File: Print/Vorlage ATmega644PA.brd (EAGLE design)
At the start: 84 x 45 mm, 58 parts, among them IC1 ATmega644PA, IC4 ATTINY24/44/84-SSU, Q1 16MHz

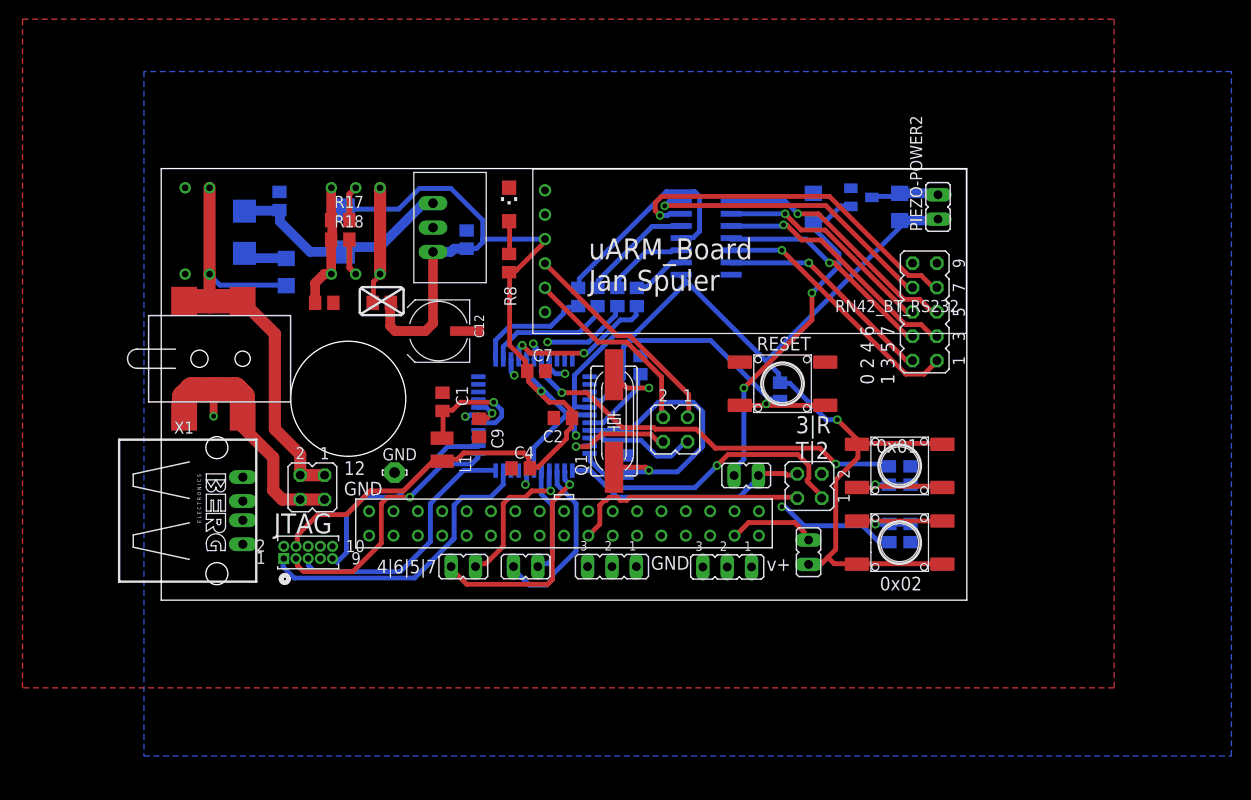
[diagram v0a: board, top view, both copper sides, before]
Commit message: print fertig
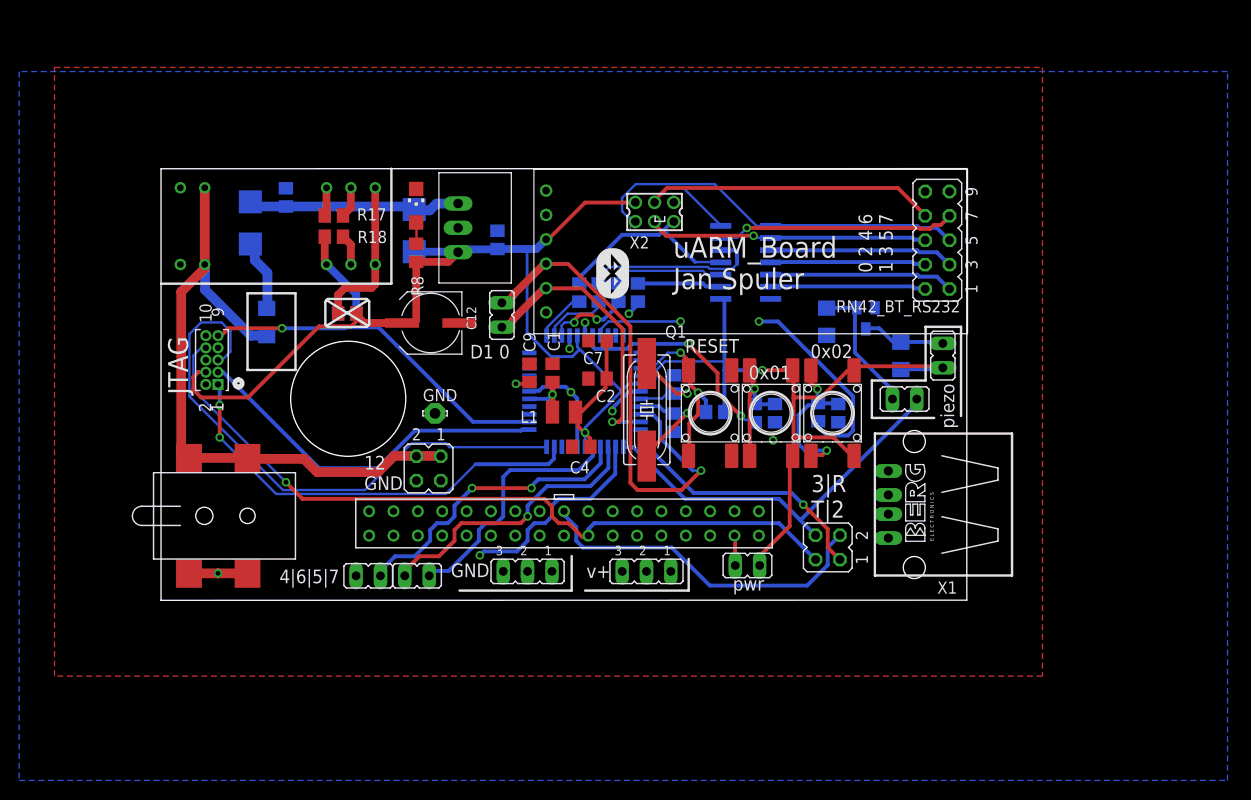
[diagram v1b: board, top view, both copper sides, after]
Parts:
- removed JP2: (no value), jumper:JP2Q
- added PIEZO-POWER6: (no value), jumper:JP1
- added X2: 87758-0616, con-molex:87758-0616
- R17, R18: value 150R -> 1k472
- moved X1 72.7 mm to (78.5, 9.97), turned to 90 degrees
- moved JTAG 25.6 mm to (4.65, 27.6), turned to 90 degrees
- moved PIEZO-POWER1 18.3 mm to (77.5, 21.0)
- moved U$1 16.4 mm to (14.0, 8.79)
- moved R3 15.6 mm to (64.0, 19.5), turned to 90 degrees
- moved R21 15.5 mm to (77.1, 25.5)
- moved PIEZO-POWER2 15.5 mm to (81.5, 25.5)
- moved R1 15.4 mm to (61.9, 19.5), turned to 90 degrees
- moved S2 15.2 mm to (70.0, 19.5), turned to 90 degrees
- moved R2 14.6 mm to (68.5, 19.6)
- moved R4 14.6 mm to (70.6, 19.5)
- moved S1 14.5 mm to (63.6, 19.5), turned to 90 degrees
- moved L1 13.3 mm to (42.0, 19.6), turned to 180 degrees
- moved V12 12.6 mm to (73.5, 29.4), turned to 180 degrees
- moved JP3 12.3 mm to (27.9, 13.7)
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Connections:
- net N$5 renamed PB2_
- net N$6 renamed PB1_
- net N$7 renamed PB0_
- removed net N$14: JP2.3, RN1.5
- removed net N$15: JP2.1, RN1.4
- removed net N$3: IC4.4, R10.2
- new net PB3_: IC4.4, R10.2, X2.5
- net GND: now also X2.6
- net PA4_: now also X2.3
- net PA5_: now also X2.1
- net PA6_: now also X2.4
- net PD0: now also PIEZO-POWER6.2, RN1.4; no longer JP2.2
- net PD1: now also PIEZO-POWER6.1, RN1.5; no longer JP2.4
- net VCC: now also X2.2
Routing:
- net PD0: track 11.9 -> 52.5 mm, vias 0 -> 1
- net VCC: track 233.4 -> 193.7 mm
- net PC3: track 27.2 -> 58.9 mm
- net N$3: track 23.3 -> 0.00 mm
- net N$15: track 23.1 -> 0.00 mm
- net RX: track 62.0 -> 84.9 mm
- net PD8: track 37.0 -> 14.4 mm, vias 2 -> 0
- net N$14: track 20.4 -> 0.00 mm
- net PB3_: track 0.00 -> 20.3 mm
- net TX: track 59.8 -> 79.6 mm, vias 0 -> 1
- net PB0: track 41.7 -> 22.9 mm
- net N$36: track 30.1 -> 11.5 mm
- net +12V: track 49.9 -> 68.2 mm
- net PD1: track 11.4 -> 29.7 mm
- net RESET: track 36.8 -> 19.6 mm, vias 1 -> 2
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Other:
- board text added: "C:/Users/Jan Spuler/OneDrive - MSW-Winterthur/Desktop/bt.bmp"
- board text added: "D1 0"
- board text added: "piezo"
- board text added: "pwr"
